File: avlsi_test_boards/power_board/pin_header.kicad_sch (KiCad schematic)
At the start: 1 part

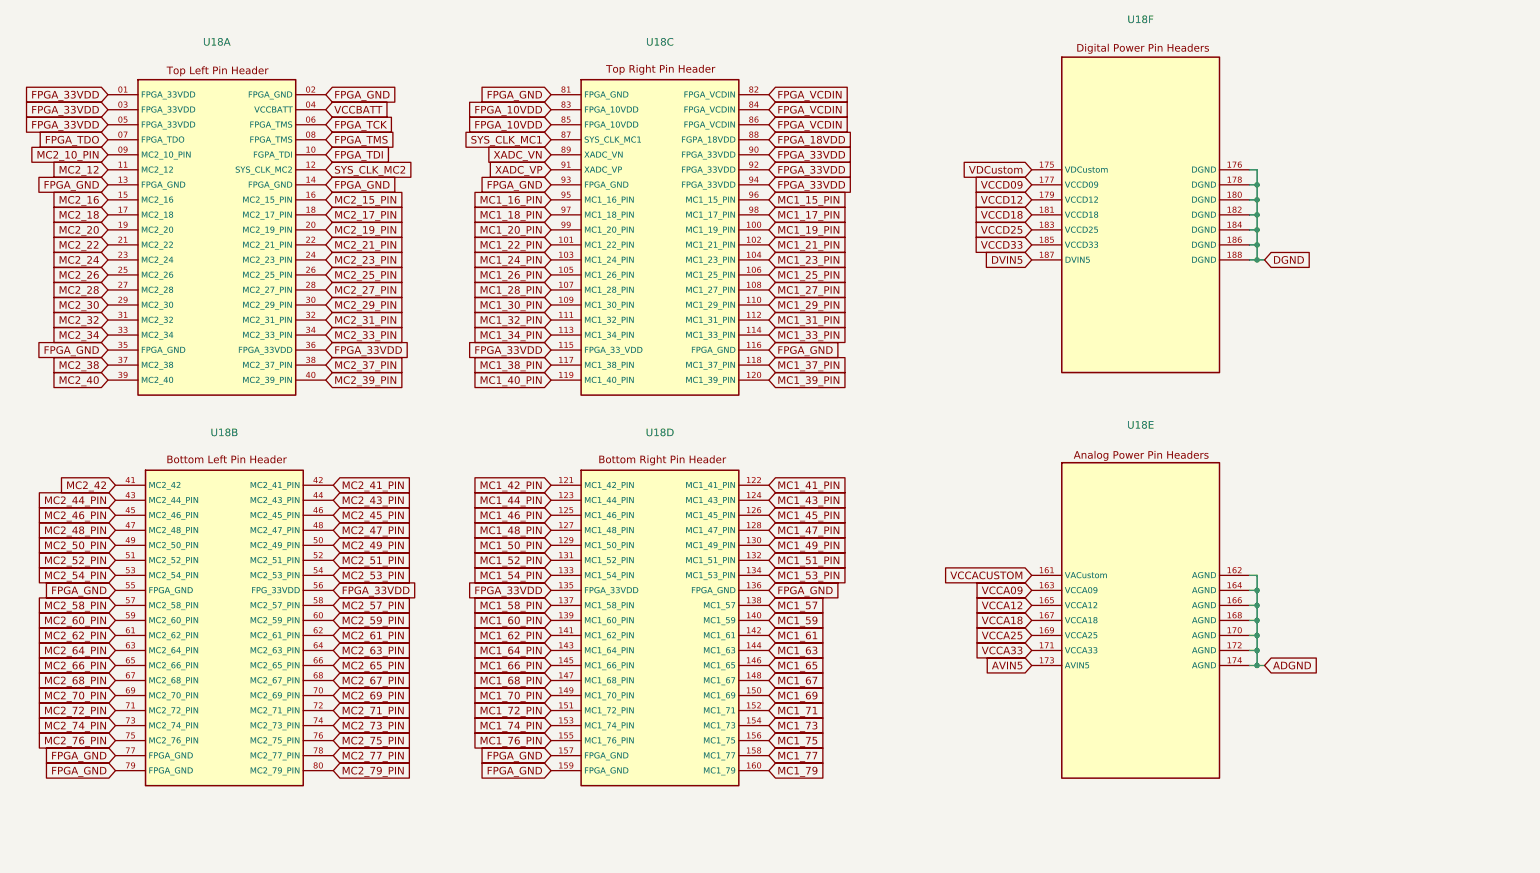
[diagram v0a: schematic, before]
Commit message: Update schematic
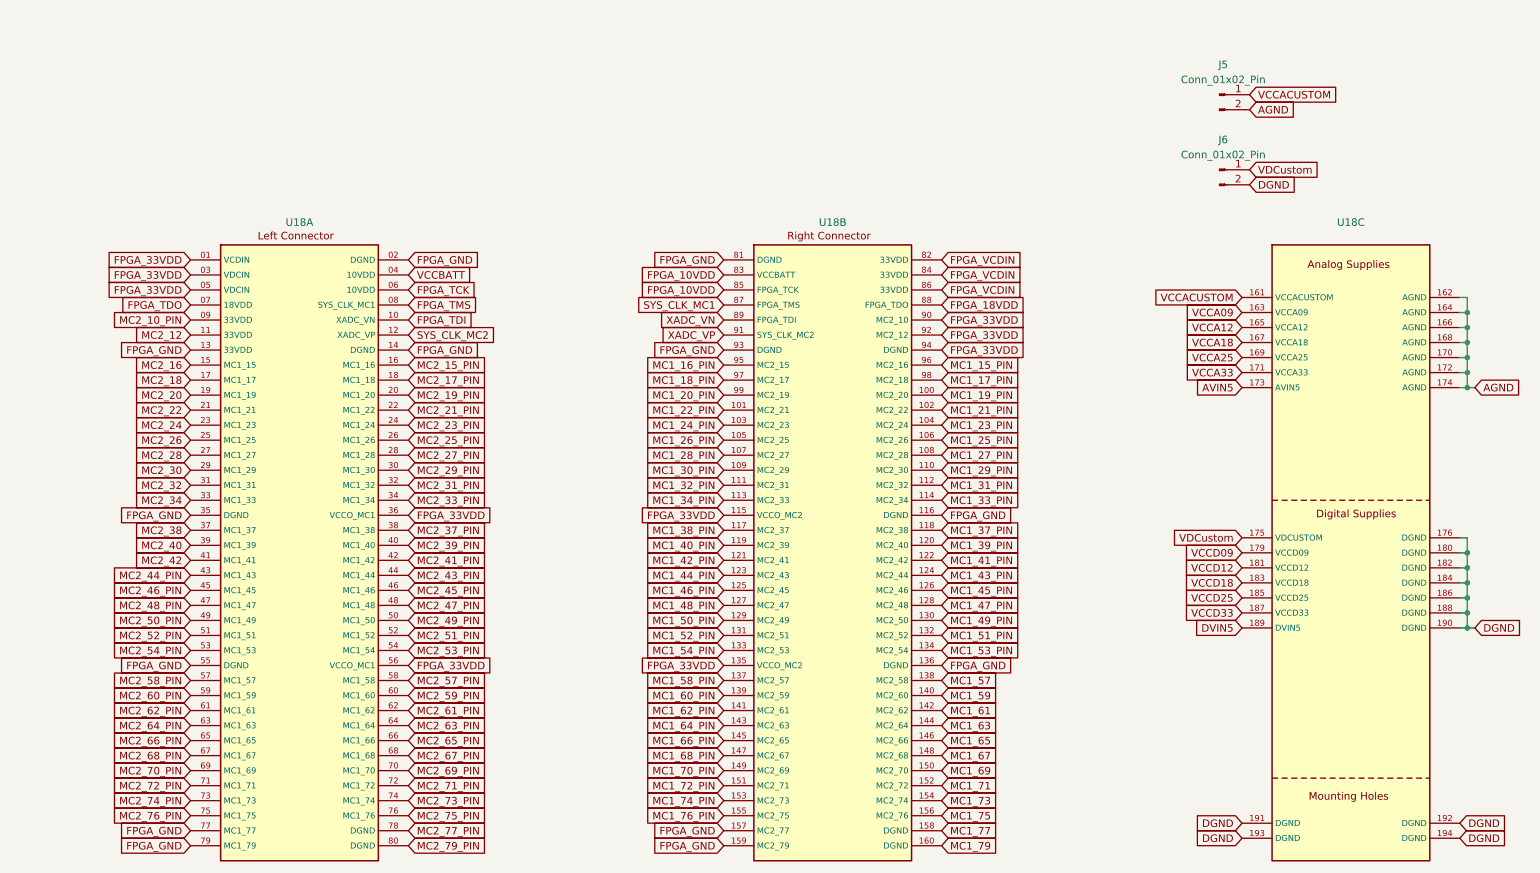
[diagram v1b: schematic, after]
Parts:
- removed U18: ~, avlsi_preferred_parts:avlsi_power_board_opal_kelly, symbol avlsi_preferred_parts:avlsi_power_board_opal_kelly
- added J5, J6: Conn_01x02_Pin, Connector_PinHeader_2.54mm:PinHeader_1x02_P2.54mm_Horizontal, symbol Connector:Conn_01x02_Pin
- added U18: ~, avlsi_preferred_parts:power_board, symbol avlsi_preferred_parts:Power_Board
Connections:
- net AVIN5: now also U18.173 (AVIN5)
- net DGND: now also J6.2 (Pin_2), U18.176 (DGND), U18.180 (DGND), U18.182 (DGND), U18.184 (DGND), U18.186 (DGND), U18.188 (DGND), U18.190 (DGND), U18.191 (DGND), U18.192 (DGND), U18.193 (DGND), U18.194 (DGND)
- net DVIN5: now also U18.189 (DVIN5)
- net FPGA_10VDD: now also U18.83 (VCCBATT), U18.85 (FPGA_TCK)
- net FPGA_18VDD: now also U18.88 (FPGA_TDO)
- net FPGA_33VDD: now also U18.01 (VCDIN), U18.03 (VDCIN), U18.05 (VDCIN), U18.115 (VCCO_MC2), U18.135 (VCCO_MC2), U18.36 (VCCO_MC1), U18.56 (VCCO_MC1), U18.90 (MC2_10), U18.92 (MC2_12), U18.94 (DGND)
- net FPGA_GND: now also U18.02 (DGND), U18.116 (DGND), U18.13 (33VDD), U18.136 (DGND), U18.14 (DGND), U18.157 (MC2_77), U18.159 (MC2_79), U18.35 (DGND), U18.55 (DGND), U18.77 (MC1_77), U18.79 (MC1_79), U18.81 (DGND), U18.93 (DGND)
- net FPGA_TCK: now also U18.06 (10VDD)
- net FPGA_TDI: now also U18.10 (XADC_VN)
- net FPGA_TDO: now also U18.07 (18VDD)
- net FPGA_TMS: now also U18.08 (SYS_CLK_MC1)
- net FPGA_VCDIN: now also U18.82 (33VDD), U18.84 (33VDD), U18.86 (33VDD)
- net MC1_15_PIN: now also U18.96 (MC2_16)
- net MC1_16_PIN: now also U18.95 (MC2_15)
- net MC1_17_PIN: now also U18.98 (MC2_18)
- net MC1_18_PIN: now also U18.97 (MC2_17)
- net MC1_19_PIN: now also U18.100 (MC2_20)
- net MC1_20_PIN: now also U18.99 (MC2_19)
- net MC1_21_PIN: now also U18.102 (MC2_22)
- net MC1_22_PIN: now also U18.101 (MC2_21)
- net MC1_23_PIN: now also U18.104 (MC2_24)
- net MC1_24_PIN: now also U18.103 (MC2_23)
- net MC1_25_PIN: now also U18.106 (MC2_26)
- net MC1_26_PIN: now also U18.105 (MC2_25)
- net MC1_27_PIN: now also U18.108 (MC2_28)
- net MC1_28_PIN: now also U18.107 (MC2_27)
- net MC1_29_PIN: now also U18.110 (MC2_30)
- net MC1_30_PIN: now also U18.109 (MC2_29)
- net MC1_31_PIN: now also U18.112 (MC2_32)
- net MC1_32_PIN: now also U18.111 (MC2_31)
- net MC1_33_PIN: now also U18.114 (MC2_34)
- net MC1_34_PIN: now also U18.113 (MC2_33)
- net MC1_37_PIN: now also U18.118 (MC2_38)
- net MC1_38_PIN: now also U18.117 (MC2_37)
- net MC1_39_PIN: now also U18.120 (MC2_40)
- net MC1_40_PIN: now also U18.119 (MC2_39)
- net MC1_41_PIN: now also U18.122 (MC2_42)
- net MC1_42_PIN: now also U18.121 (MC2_41)
- net MC1_43_PIN: now also U18.124 (MC2_44)
- net MC1_44_PIN: now also U18.123 (MC2_43)
- net MC1_45_PIN: now also U18.126 (MC2_46)
- net MC1_46_PIN: now also U18.125 (MC2_45)
- net MC1_47_PIN: now also U18.128 (MC2_48)
- net MC1_48_PIN: now also U18.127 (MC2_47)
- net MC1_49_PIN: now also U18.130 (MC2_50)
- net MC1_50_PIN: now also U18.129 (MC2_49)
- net MC1_51_PIN: now also U18.132 (MC2_52)
- net MC1_52_PIN: now also U18.131 (MC2_51)
- net MC1_53_PIN: now also U18.134 (MC2_54)
- net MC1_54_PIN: now also U18.133 (MC2_53)
- net MC1_57: now also U18.138 (MC2_58)
- net MC1_58_PIN: now also U18.137 (MC2_57)
- net MC1_59: now also U18.140 (MC2_60)
- net MC1_60_PIN: now also U18.139 (MC2_59)
- net MC1_61: now also U18.142 (MC2_62)
- net MC1_62_PIN: now also U18.141 (MC2_61)
- net MC1_63: now also U18.144 (MC2_64)
- net MC1_64_PIN: now also U18.143 (MC2_63)
- net MC1_65: now also U18.146 (MC2_66)
- net MC1_66_PIN: now also U18.145 (MC2_65)
- net MC1_67: now also U18.148 (MC2_68)
- net MC1_68_PIN: now also U18.147 (MC2_67)
- net MC1_69: now also U18.150 (MC2_70)
- net MC1_70_PIN: now also U18.149 (MC2_69)
- net MC1_71: now also U18.152 (MC2_72)
- net MC1_72_PIN: now also U18.151 (MC2_71)
- net MC1_73: now also U18.154 (MC2_74)
- net MC1_74_PIN: now also U18.153 (MC2_73)
- net MC1_75: now also U18.156 (MC2_76)
- net MC1_76_PIN: now also U18.155 (MC2_75)
- net MC1_77: now also U18.158 (DGND)
- net MC1_79: now also U18.160 (DGND)
- net MC2_10_PIN: now also U18.09 (33VDD)
- net MC2_12: now also U18.11 (33VDD)
- net MC2_15_PIN: now also U18.16 (MC1_16)
- net MC2_16: now also U18.15 (MC1_15)
- net MC2_17_PIN: now also U18.18 (MC1_18)
- net MC2_18: now also U18.17 (MC1_17)
- net MC2_19_PIN: now also U18.20 (MC1_20)
- net MC2_20: now also U18.19 (MC1_19)
- net MC2_21_PIN: now also U18.22 (MC1_22)
- net MC2_22: now also U18.21 (MC1_21)
- net MC2_23_PIN: now also U18.24 (MC1_24)
- net MC2_24: now also U18.23 (MC1_23)
- net MC2_25_PIN: now also U18.26 (MC1_26)
- net MC2_26: now also U18.25 (MC1_25)
- net MC2_27_PIN: now also U18.28 (MC1_28)
- net MC2_28: now also U18.27 (MC1_27)
- net MC2_29_PIN: now also U18.30 (MC1_30)
- net MC2_30: now also U18.29 (MC1_29)
- net MC2_31_PIN: now also U18.32 (MC1_32)
- net MC2_32: now also U18.31 (MC1_31)
- net MC2_33_PIN: now also U18.34 (MC1_34)
- net MC2_34: now also U18.33 (MC1_33)
- net MC2_37_PIN: now also U18.38 (MC1_38)
- net MC2_38: now also U18.37 (MC1_37)
- net MC2_39_PIN: now also U18.40 (MC1_40)
- net MC2_40: now also U18.39 (MC1_39)
- net MC2_41_PIN: now also U18.42 (MC1_42)
- net MC2_42: now also U18.41 (MC1_41)
- net MC2_43_PIN: now also U18.44 (MC1_44)
- net MC2_44_PIN: now also U18.43 (MC1_43)
- net MC2_45_PIN: now also U18.46 (MC1_46)
- net MC2_46_PIN: now also U18.45 (MC1_45)
- net MC2_47_PIN: now also U18.48 (MC1_48)
- net MC2_48_PIN: now also U18.47 (MC1_47)
- net MC2_49_PIN: now also U18.50 (MC1_50)
- net MC2_50_PIN: now also U18.49 (MC1_49)
- net MC2_51_PIN: now also U18.52 (MC1_52)
- net MC2_52_PIN: now also U18.51 (MC1_51)
- net MC2_53_PIN: now also U18.54 (MC1_54)
- net MC2_54_PIN: now also U18.53 (MC1_53)
- net MC2_57_PIN: now also U18.58 (MC1_58)
- net MC2_58_PIN: now also U18.57 (MC1_57)
- net MC2_59_PIN: now also U18.60 (MC1_60)
- net MC2_60_PIN: now also U18.59 (MC1_59)
- net MC2_61_PIN: now also U18.62 (MC1_62)
- net MC2_62_PIN: now also U18.61 (MC1_61)
- net MC2_63_PIN: now also U18.64 (MC1_64)
- net MC2_64_PIN: now also U18.63 (MC1_63)
- net MC2_65_PIN: now also U18.66 (MC1_66)
- net MC2_66_PIN: now also U18.65 (MC1_65)
- net MC2_67_PIN: now also U18.68 (MC1_68)
- net MC2_68_PIN: now also U18.67 (MC1_67)
- net MC2_69_PIN: now also U18.70 (MC1_70)
- net MC2_70_PIN: now also U18.69 (MC1_69)
- net MC2_71_PIN: now also U18.72 (MC1_72)
- net MC2_72_PIN: now also U18.71 (MC1_71)
- net MC2_73_PIN: now also U18.74 (MC1_74)
- net MC2_74_PIN: now also U18.73 (MC1_73)
- net MC2_75_PIN: now also U18.76 (MC1_76)
- net MC2_76_PIN: now also U18.75 (MC1_75)
- net MC2_77_PIN: now also U18.78 (DGND)
- net MC2_79_PIN: now also U18.80 (DGND)
- net SYS_CLK_MC1: now also U18.87 (FPGA_TMS)
- net SYS_CLK_MC2: now also U18.12 (XADC_VP)
- net VCCA09: now also U18.163 (VCCA09)
- net VCCA12: now also U18.165 (VCCA12)
- net VCCA18: now also U18.167 (VCCA18)
- net VCCA25: now also U18.169 (VCCA25)
- net VCCA33: now also U18.171 (VCCA33)
- net VCCACUSTOM: now also J5.1 (Pin_1), U18.161 (VCCACUSTOM)
- net VCCBATT: now also U18.04 (10VDD)
- net VCCD09: now also U18.179 (VCCD09)
- net VCCD12: now also U18.181 (VCCD12)
- net VCCD18: now also U18.183 (VCCD18)
- net VCCD25: now also U18.185 (VCCD25)
- net VCCD33: now also U18.187 (VCCD33)
- net VDCustom: now also J6.1 (Pin_1), U18.175 (VDCUSTOM)
- net XADC_VN: now also U18.89 (FPGA_TDI)
- net XADC_VP: now also U18.91 (SYS_CLK_MC2)
- new net AGND: J5.2 (Pin_2), U18.162 (AGND), U18.164 (AGND), U18.166 (AGND), U18.168 (AGND), U18.170 (AGND), U18.172 (AGND), U18.174 (AGND)
